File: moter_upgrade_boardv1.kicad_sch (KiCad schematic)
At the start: 51 parts, among them J1 Conn_01x04_Socket, J2 Conn_01x03_Socket, J3 Conn_01x02_Socket, J4 Conn_01x03_Socket, J5 Conn_01x05_Socket, J6 USB_C_Receptacle_USB2.0_16P, SW1 SW_SPDT, SW2 SW_Push, SW3 SW_Wuerth_450301014042, U1 BD33FC0FP, U2 TLP785, U3 TLP785, U4 STM32H523CCTx, U5 MCP2562-E-P, U6 CH340E, U7 BD33FC0FP

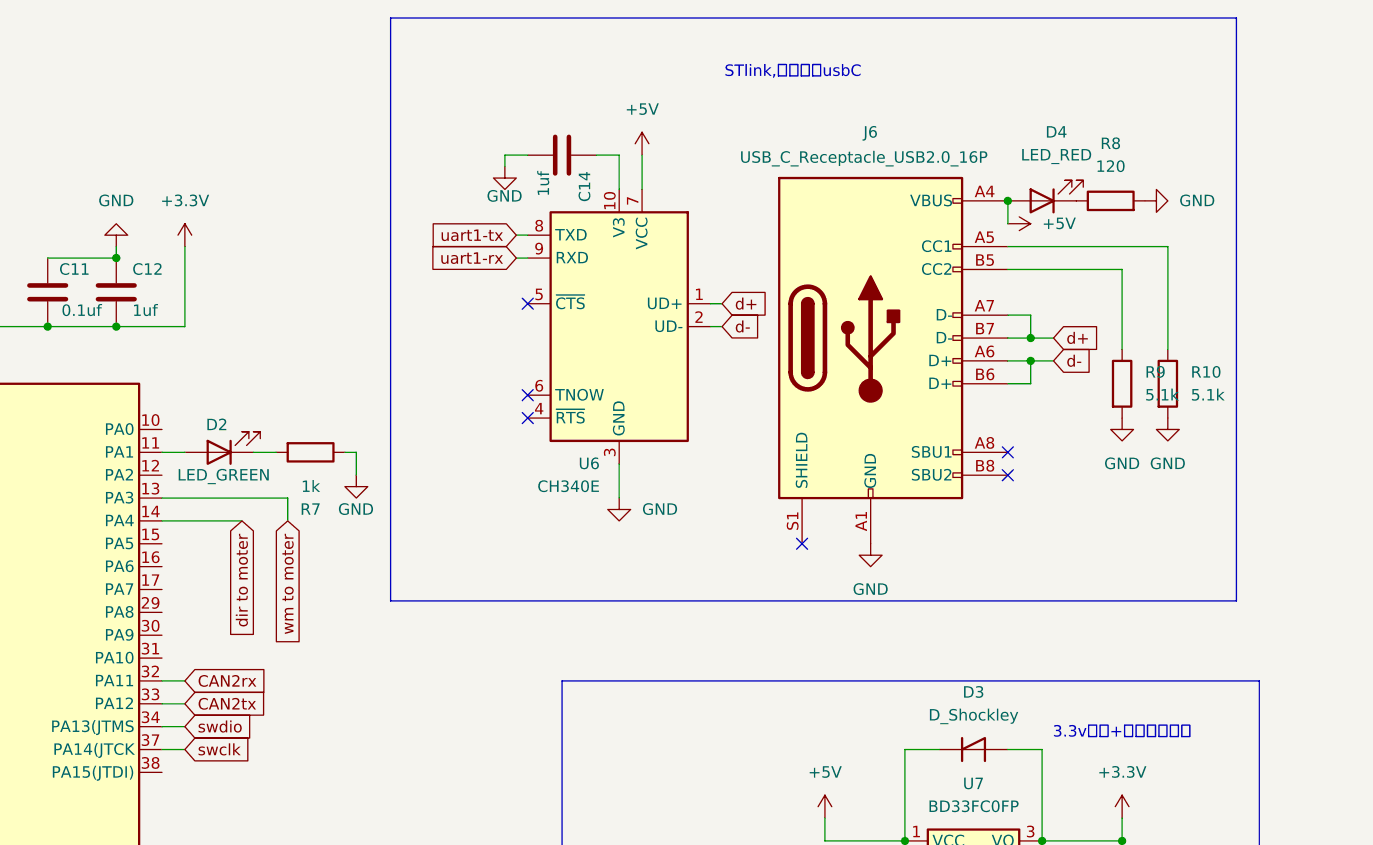
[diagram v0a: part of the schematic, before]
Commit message: 配線、配置変更など　いったん完成
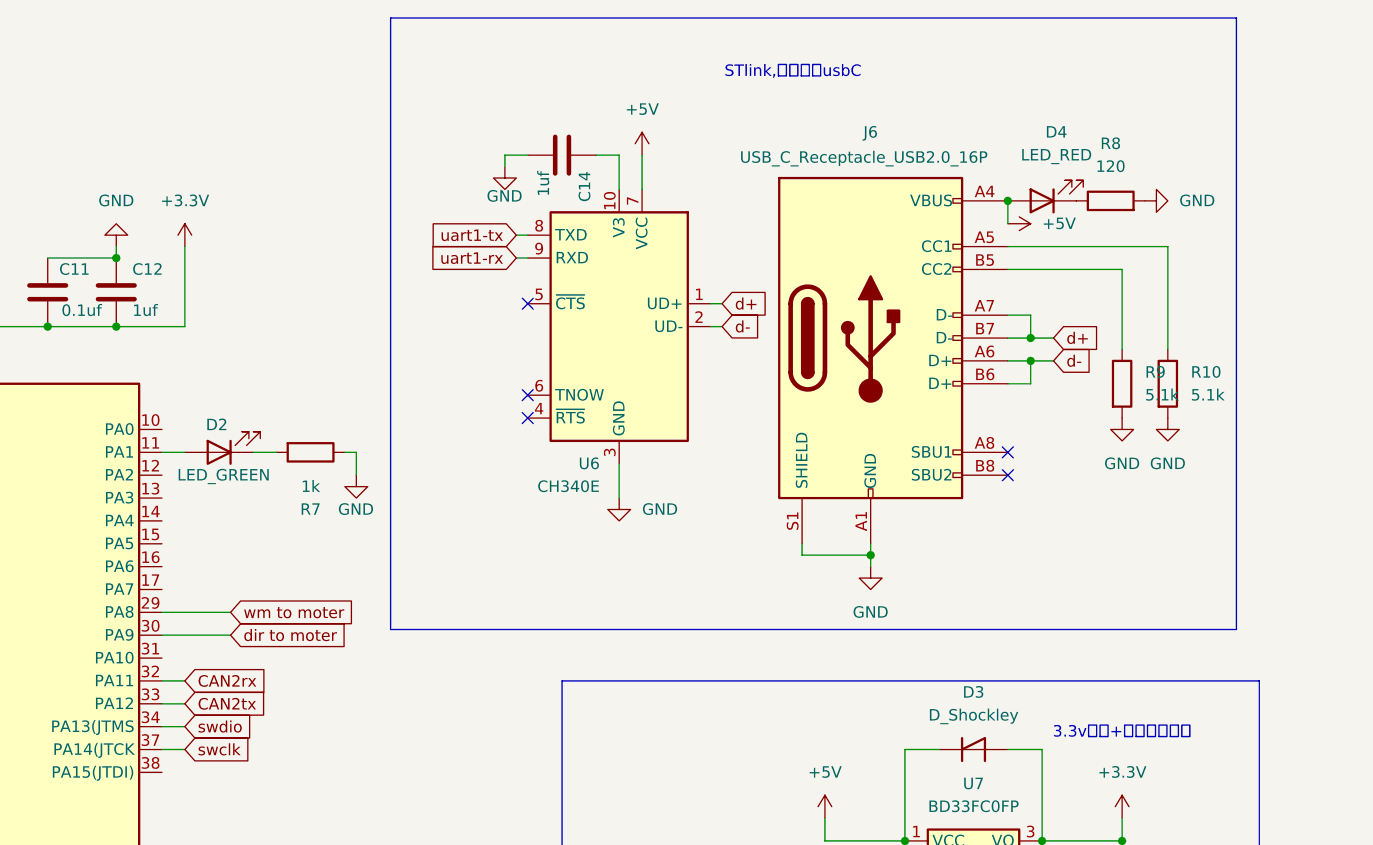
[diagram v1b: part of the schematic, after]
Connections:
- net GND: now also J6.S1 (SHIELD)
- net dir to moter: now also U4.30 (PA9); no longer U4.14 (PA4)
- net wm to moter: now also U4.29 (PA8); no longer U4.13 (PA3)
- no-connect marks 8 -> 7
